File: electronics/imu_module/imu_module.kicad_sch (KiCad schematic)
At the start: 36 parts, among them J1 Conn_01x06_Male, J2 Conn_01x04_Pin, J3 Conn_01x04, J4 Conn_01x04, SW1 SW_Push, SW2 SW_Push, SW3 SW_Push, U1 ESP32-WROOM-32U, U2 BMI088, U3 SN74LV1T34DBV, U4 SP485, U5 AP2114HA-3.3TRG1

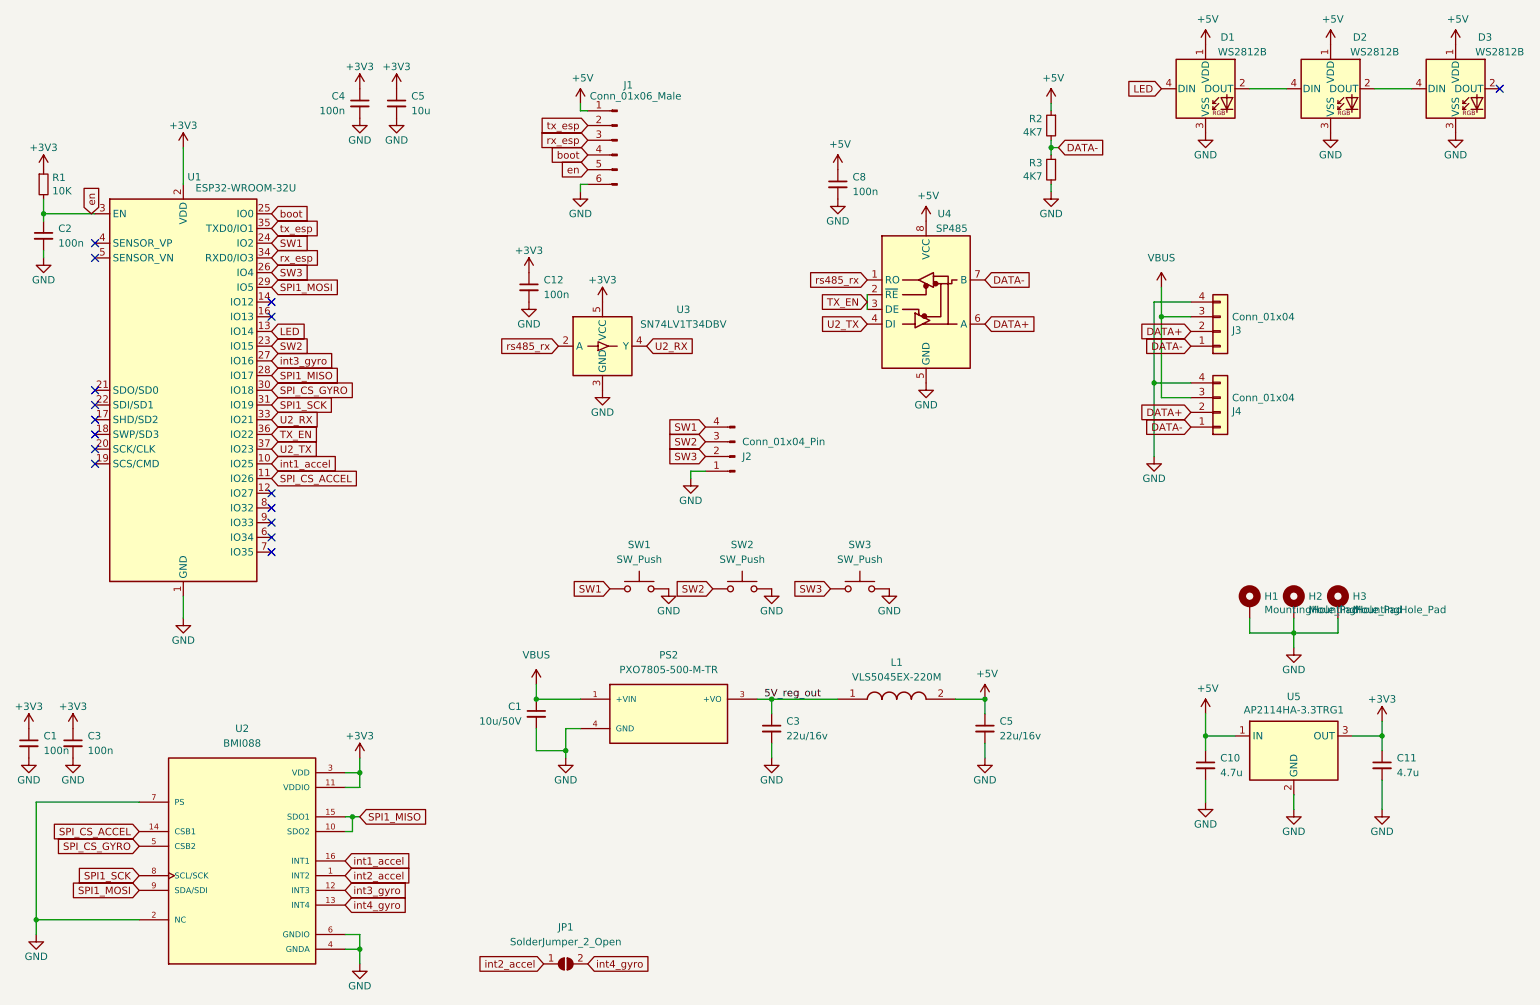
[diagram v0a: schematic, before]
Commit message: production version and bom
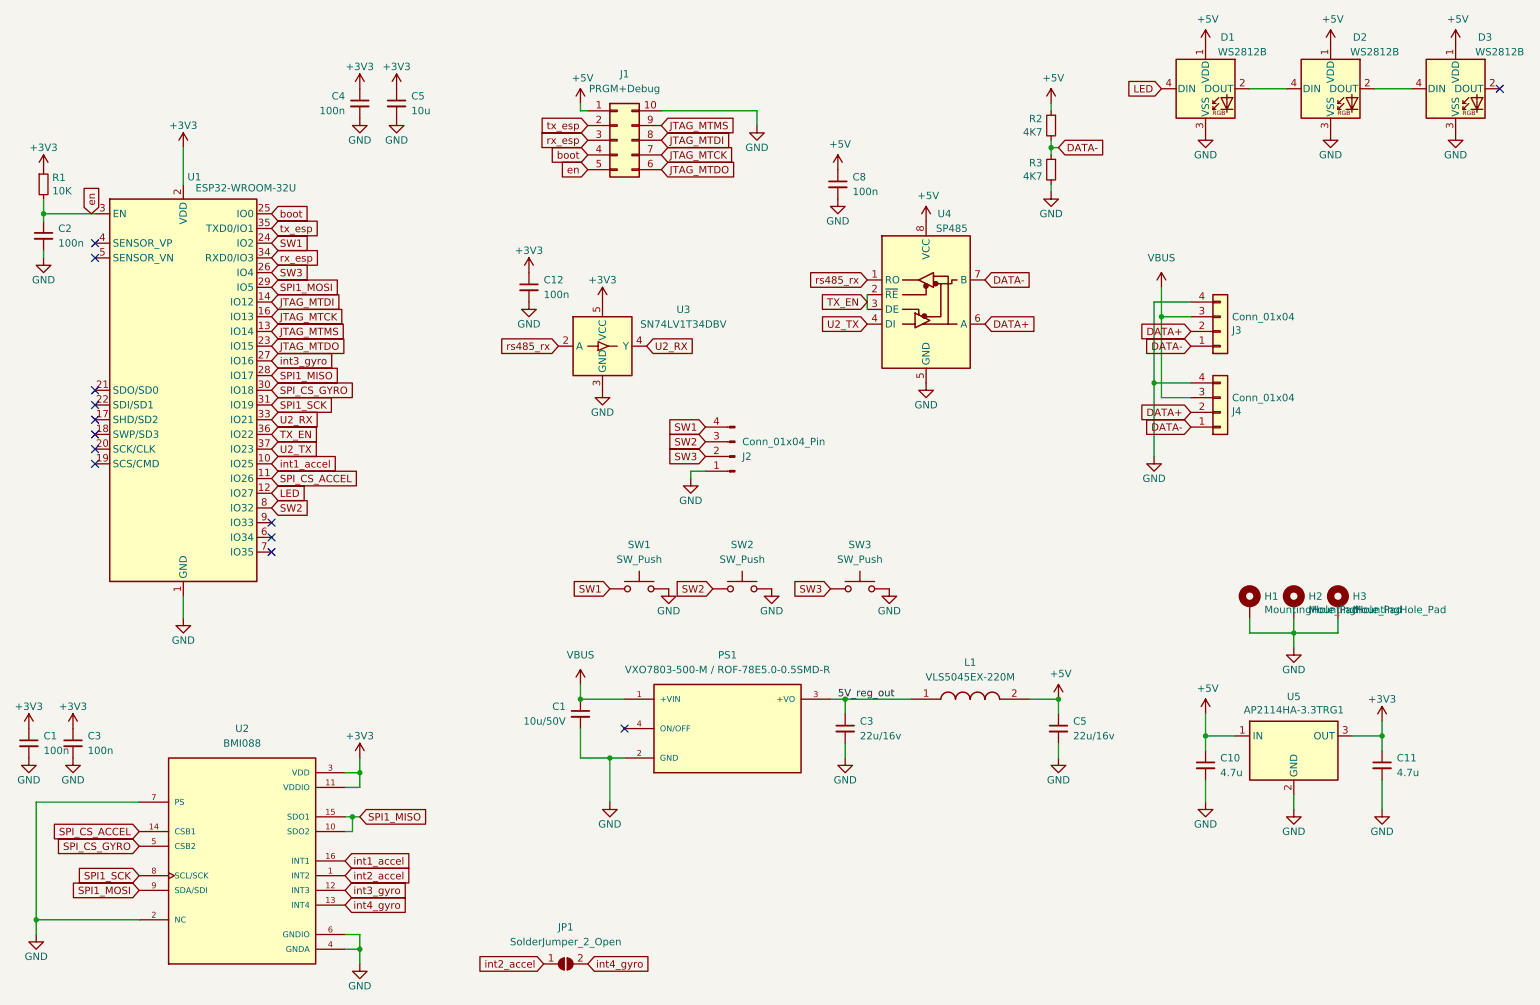
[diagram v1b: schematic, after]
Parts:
- removed J1: Conn_01x06_Male, lib:esp32_pogo_programmer, symbol Connector:Conn_01x06_Male
- removed PS2: PXO7805-500-M-TR, lib:PXO7805-500-M-TR, symbol PXO7805-500-M-TR:PXO7805-500-M-TR
- added J1: PRGM+Debug, lib:esp32_prgm_debug, symbol Connector_Generic:Conn_02x05_Counter_Clockwise
- added PS1: VXO7803-500-M / ROF-78E5.0-0.5SMD-R, lib:CONV_VXO7803-500-M, symbol VXO:VXO7803-500-M
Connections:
- net +5V: now also J1.1 (Pin_1)
- net 5V_reg_out: now also PS1.3 (+VO)
- net GND: now also J1.10 (Pin_10), PS1.2 (GND)
- net LED: now also U1.12 (IO27); no longer U1.13 (IO14)
- net SW2: now also U1.8 (IO32); no longer U1.23 (IO15)
- net VBUS: now also PS1.1 (+VIN)
- net boot: now also J1.4 (Pin_4)
- net en: now also J1.5 (Pin_5)
- net rx_esp: now also J1.3 (Pin_3)
- net tx_esp: now also J1.2 (Pin_2)
- net JTAG_MTDI: now reaches U1.14 (IO12)
- net JTAG_MTDI: now also J1.8 (Pin_8)
- net JTAG_MTCK: now reaches U1.16 (IO13)
- net JTAG_MTCK: now also J1.7 (Pin_7)
- new net JTAG_MTDO: J1.6 (Pin_6), U1.23 (IO15)
- new net JTAG_MTMS: J1.9 (Pin_9), U1.13 (IO14)
- no-connect marks 16 -> 13
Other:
- moved on the sheet: C1, C3, C5, L1
